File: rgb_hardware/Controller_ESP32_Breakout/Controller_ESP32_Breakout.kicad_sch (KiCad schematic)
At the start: 3 parts, among them J1 Power, J2 LED Strip Driver, U1 ESP32_NODEMCU

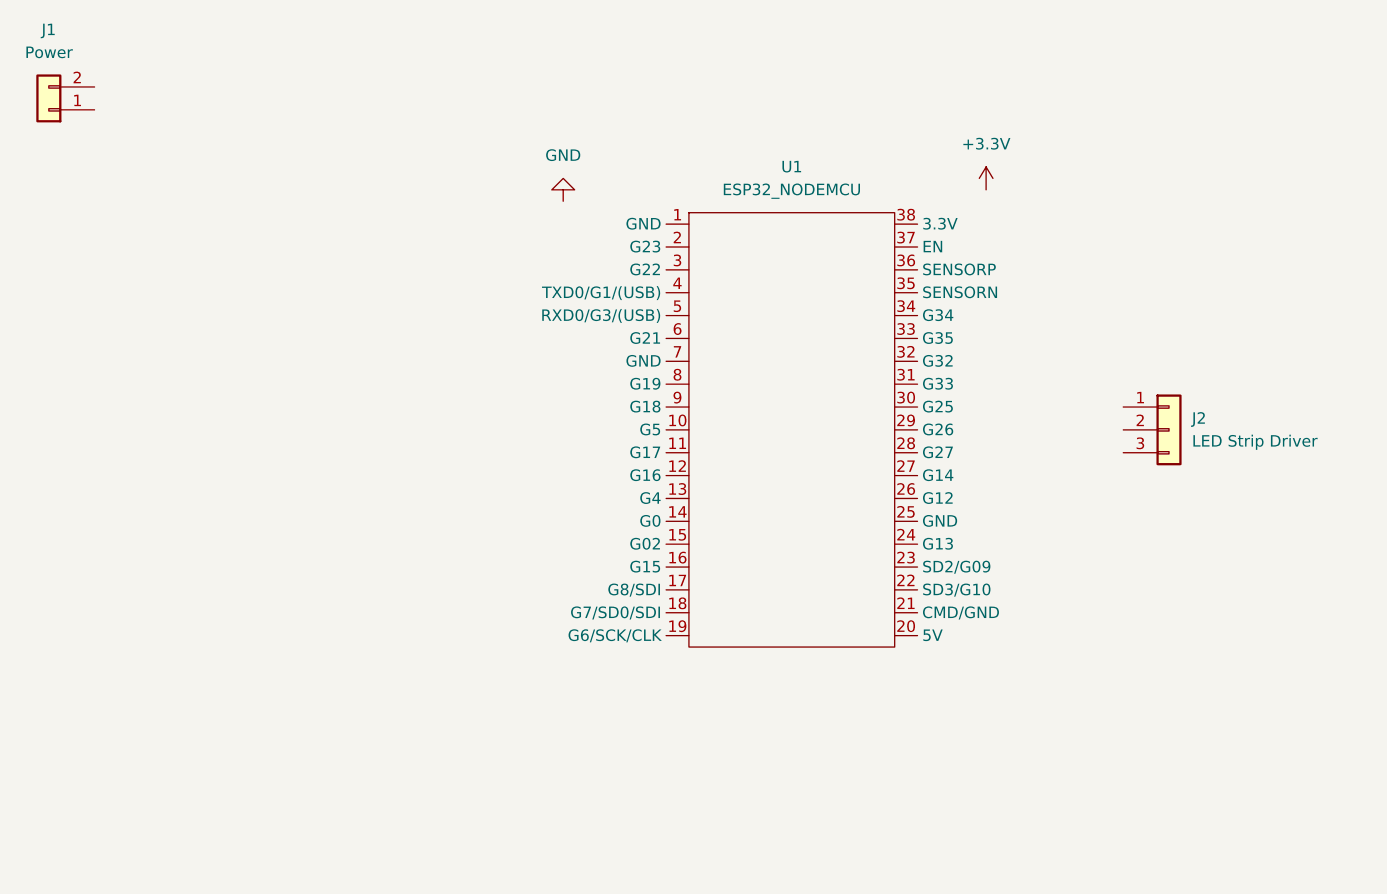
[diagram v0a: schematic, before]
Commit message: step forward with the breakout board
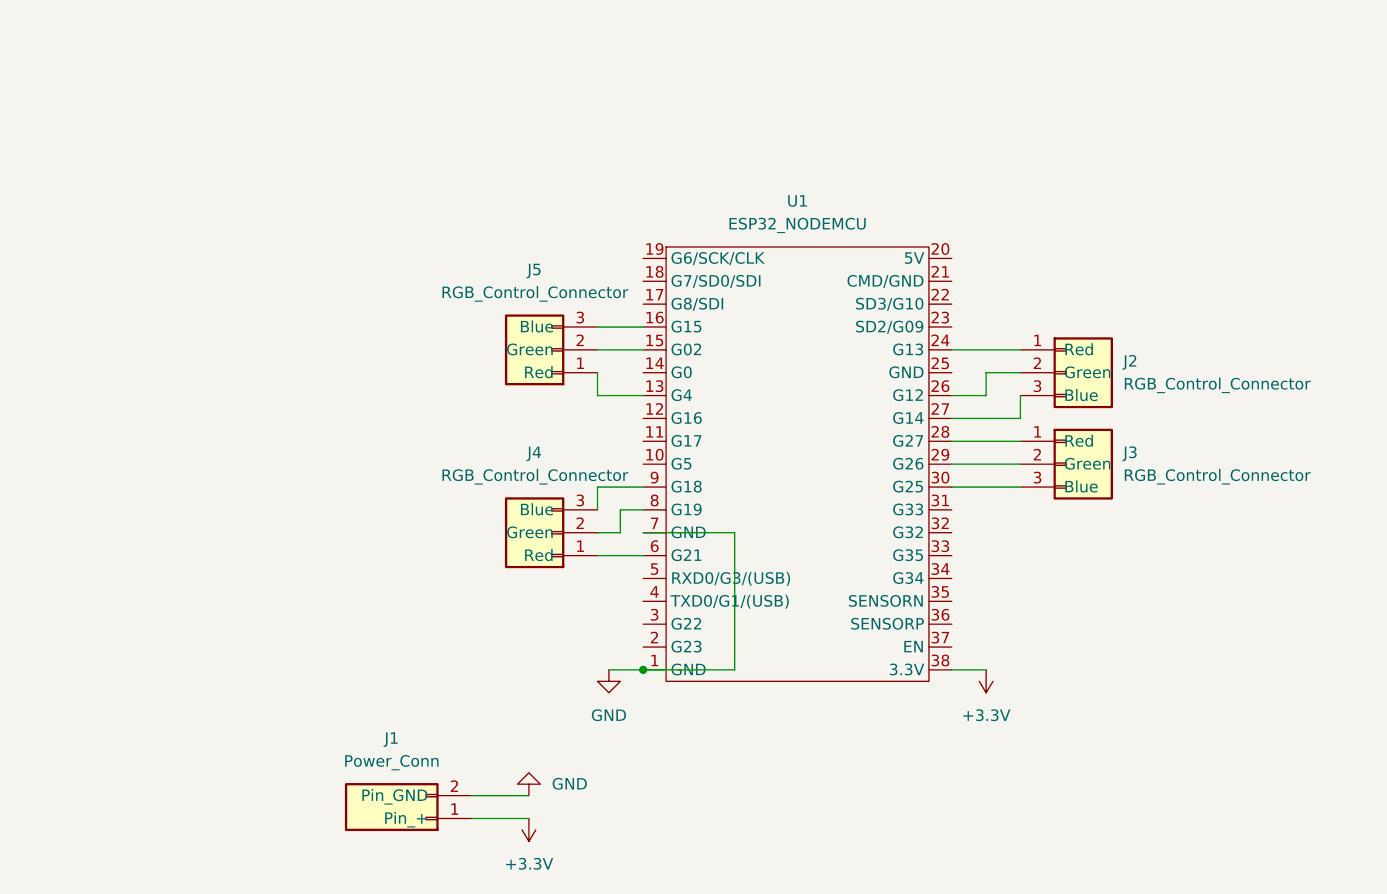
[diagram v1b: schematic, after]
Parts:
- removed J1: Power, Connector_PinHeader_2.54mm:PinHeader_1x02_P2.54mm_Horizontal, symbol Connector_Generic:Conn_01x02
- removed J2: LED Strip Driver, Connector_PinHeader_2.54mm:PinHeader_1x03_P2.54mm_Horizontal, symbol Connector_Generic:Conn_01x03
- removed U1: ESP32_NODEMCU, AC_Delivery:ESP32 NODEMCU, symbol ac_delivery:ESP32_NODEMCU
- added J1: Power_Conn, Connector_PinHeader_2.54mm:PinHeader_1x02_P2.54mm_Horizontal, symbol Connector_Project:Power_Conn
- added J2, J3, J4, J5: RGB_Control_Connector, Connector_PinHeader_2.54mm:PinHeader_1x03_P2.54mm_Horizontal, symbol Connector_Project:RGB_Control_Connector
- added U1: ESP32_NODEMCU, AZ_Delivery:ESP32 NODEMCU, symbol AZ_Delivery:ESP32_NODEMCU
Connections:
- net +3.3V: now also J1.1 (Pin_+), U1.38 (3.3V)
- net GND: now also J1.2 (Pin_GND), U1.1 (GND), U1.7 (GND)
- new net: J2.1 (Red), U1.24 (G13)
- new net: J2.2 (Green), U1.26 (G12)
- new net: J2.3 (Blue), U1.27 (G14)
- new net: J5.1 (Red), U1.13 (G4)
- new net: J5.2 (Green), U1.15 (G02)
- new net: J5.3 (Blue), U1.16 (G15)
- new net: J3.1 (Red), U1.28 (G27)
- new net: J3.2 (Green), U1.29 (G26)
- new net: J3.3 (Blue), U1.30 (G25)
- new net: J4.1 (Red), U1.6 (G21)
- new net: J4.2 (Green), U1.8 (G19)
- new net: J4.3 (Blue), U1.9 (G18)
